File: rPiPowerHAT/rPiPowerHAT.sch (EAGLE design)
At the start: 3 parts, among them X1 MKDSN1,5/2-5,08, X2 MKDSN1,5/2-5,08

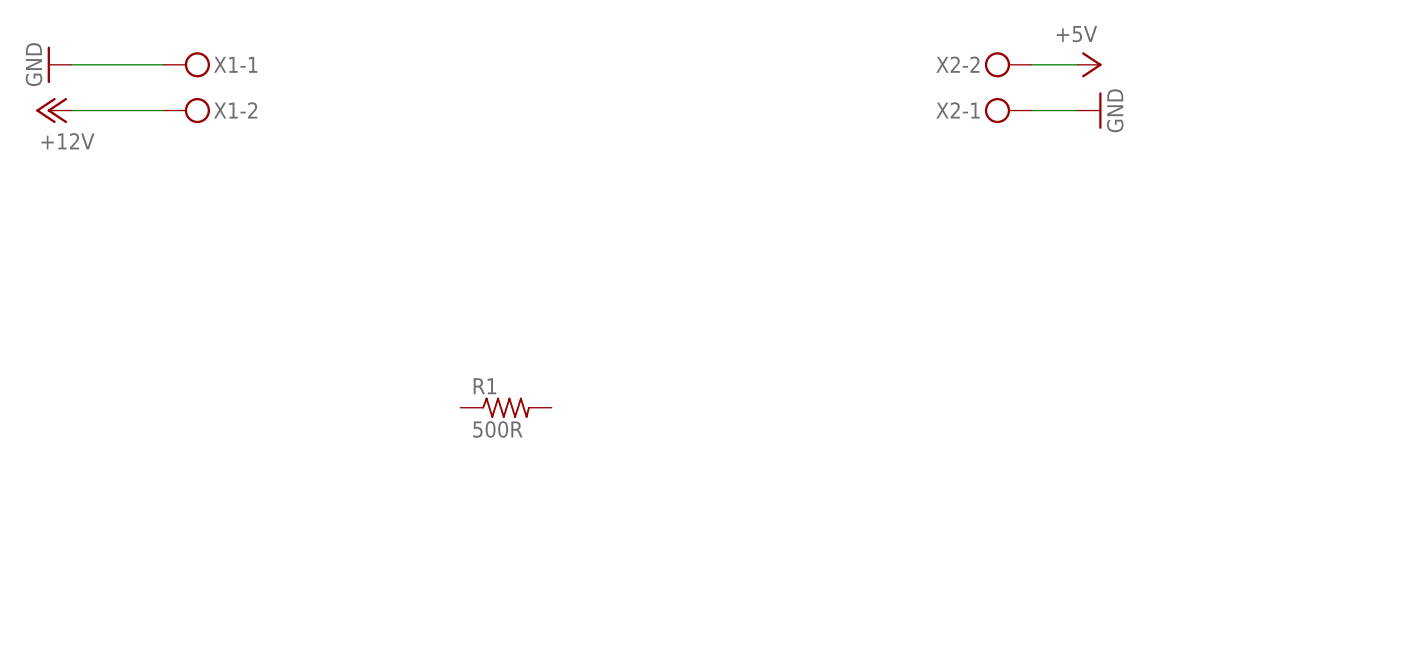
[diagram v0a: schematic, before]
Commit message: .
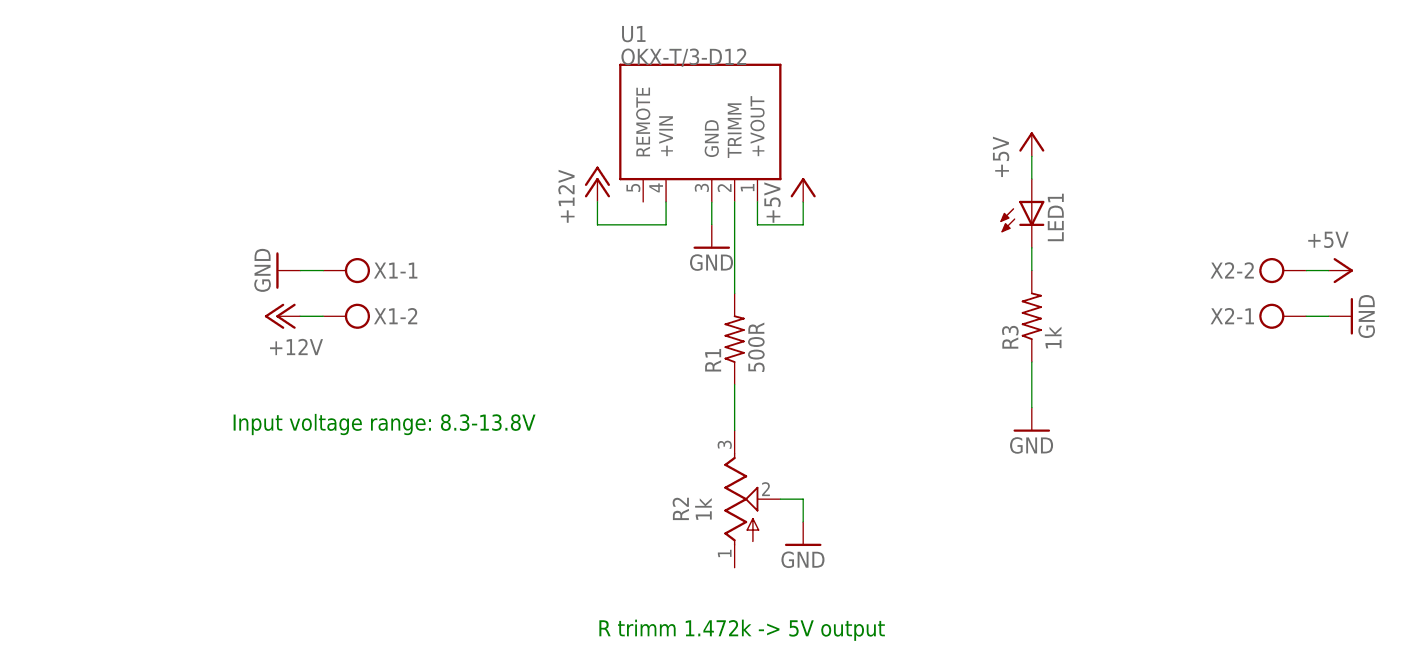
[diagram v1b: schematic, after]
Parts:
- added LED1: (no value), adafruit:LEDCHIP-LED0603
- added R2: 1k, hojunsong:POT-3296W
- added R3: 1k, rcl:R-US_R0603
- added U1: OKX-T/3-D12, hojunsong:OKX-T/3-D12
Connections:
- new net N$1: R1.2, U1.TRIMM
- new net N$2: R1.1, R2.E
- new net N$3: LED1.C, R3.2
- net +12V: now also U1.+VIN
- net +5V: now also LED1.A, U1.+VOUT
- net GND: now also R2.S, R3.1, U1.GND
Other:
- note added: "Input voltage range: 8.3-13.8V"
- note added: "R trimm 1.472k -> 5V output"
- moved on the sheet: R1, X1-1, X1-2, X2-1, X2-2
